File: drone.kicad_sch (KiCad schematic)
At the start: 0 parts

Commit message: Added sensors and mcu
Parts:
- added J1: Battery-Banana-Plug-Connector, symbol Connector_Generic:Conn_01x02
- added J10: GPIO7 TH, symbol Connector_Generic:Conn_01x01
- added J11, J12, J13, J14, J15, J16, J17, J18, J19, J20, J8: Conn_01x01, symbol Connector_Generic:Conn_01x01
- added J2: AF-MPM3610-Converter, Adafruit MPM3610:1X04_ROUND, symbol Adafruit MPM3610-eagle-import:HEADER-1X4ROUND
- added J21: GPIO9_TH, symbol Connector_Generic:Conn_01x01
- added J22: GPIO8 TH, symbol Connector_Generic:Conn_01x01
- added J3: ESC_1, symbol Connector_Generic:Conn_01x01
- added J4: ESC_2, symbol Connector_Generic:Conn_01x01
- added J5, J6: ESC_3, symbol Connector_Generic:Conn_01x01
- added J7: VCC_MCU_Sensors, symbol Connector_Generic:Conn_01x01
- added J9: GPIO44 TH, symbol Connector_Generic:Conn_01x01
- added S1: AF-QMC5883P-Magnetometer, Adafruit QMC5883P Magnetometer:1X05_ROUND_70, symbol Adafruit QMC5883P Magnetometer-eagle-import:HEADER-1X570MIL
- added S2: AF-BMP280-Barometer, Adafruit BMP280:1X07_ROUND_70, symbol Adafruit BMP280-eagle-import:HEADER-1X770MIL
- added S3: AF-MPU6050-Accel/Gyro, Adafruit MPU6050:1X06_ROUND_70, symbol Adafruit MPU6050-eagle-import:HEADER-1X670MIL
- added S4: AF-MPU6050-Accel/Gyro, Adafruit MPU6050:1X06_ROUND, symbol Adafruit MPU6050-eagle-import:HEADER-1X6ROUND
- added U1, U2: ESP32-S3, symbol Adafruit BMP280-eagle-import:HEADER-1X770MIL
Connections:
- new net: J14.1 (Pin_1), S4.4
- new net 3Vo: S1.2, S2.2, S3.2
- new net 5VIN: U1.1
- new net AD0: J11.1 (Pin_1), S4.1
- new net CLKIN: J15.1 (Pin_1), S4.5
- new net CS_5V: S2.7
- new net EN: J2.1
- new net FSYNC_IN: J12.1 (Pin_1), S4.2
- new net GND: J1.2 (Pin_2), J2.4, S1.3, S2.3, S3.3, S4.6, U1.2
- new net GPIO1: J16.1 (Pin_1), U2.1
- new net GPIO2: J17.1 (Pin_1), U2.2
- new net GPIO3: J18.1 (Pin_1), U2.3
- new net GPIO4: J19.1 (Pin_1), U2.4
- new net GPIO43: J20.1 (Pin_1), S1.4, S2.4, S3.4, U2.6, U2.7
- new net GPIO44: J9.1 (Pin_1), U1.7
- new net GPIO7: J10.1 (Pin_1), U1.6
- new net GPIO8: J22.1 (Pin_1), U1.5
- new net GPIO9: J21.1 (Pin_1), U1.4
- new net INT: S3.6
- new net SCL_EXT: J13.1 (Pin_1), S4.3
- new net SDA: S1.5, S2.6, S3.5, U2.5
- new net SDO/ADR_3V: S2.5
- new net VBat: J1.1 (Pin_1), J2.2, J3.1 (Pin_1), J4.1 (Pin_1), J5.1 (Pin_1), J6.1 (Pin_1)
- new net VCC_3V3: J2.3, J8.1 (Pin_1)
- new net VCC_3V3_MCU: J7.1 (Pin_1), S1.1, S2.1, S3.1, U1.3

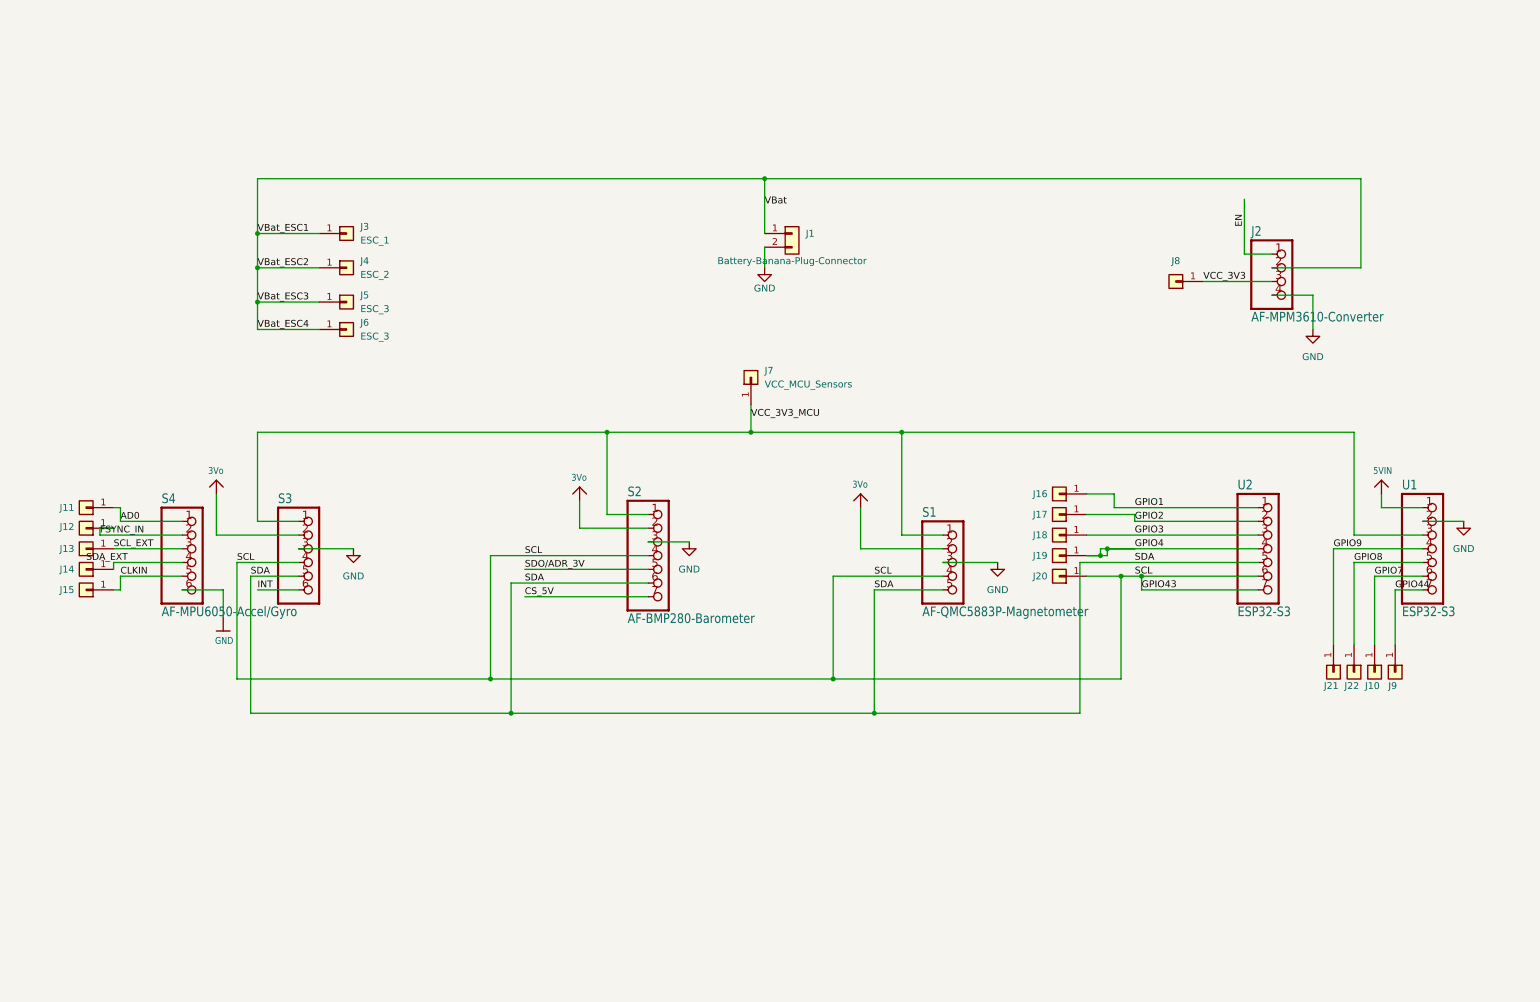
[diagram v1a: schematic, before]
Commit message: Initial commit 2
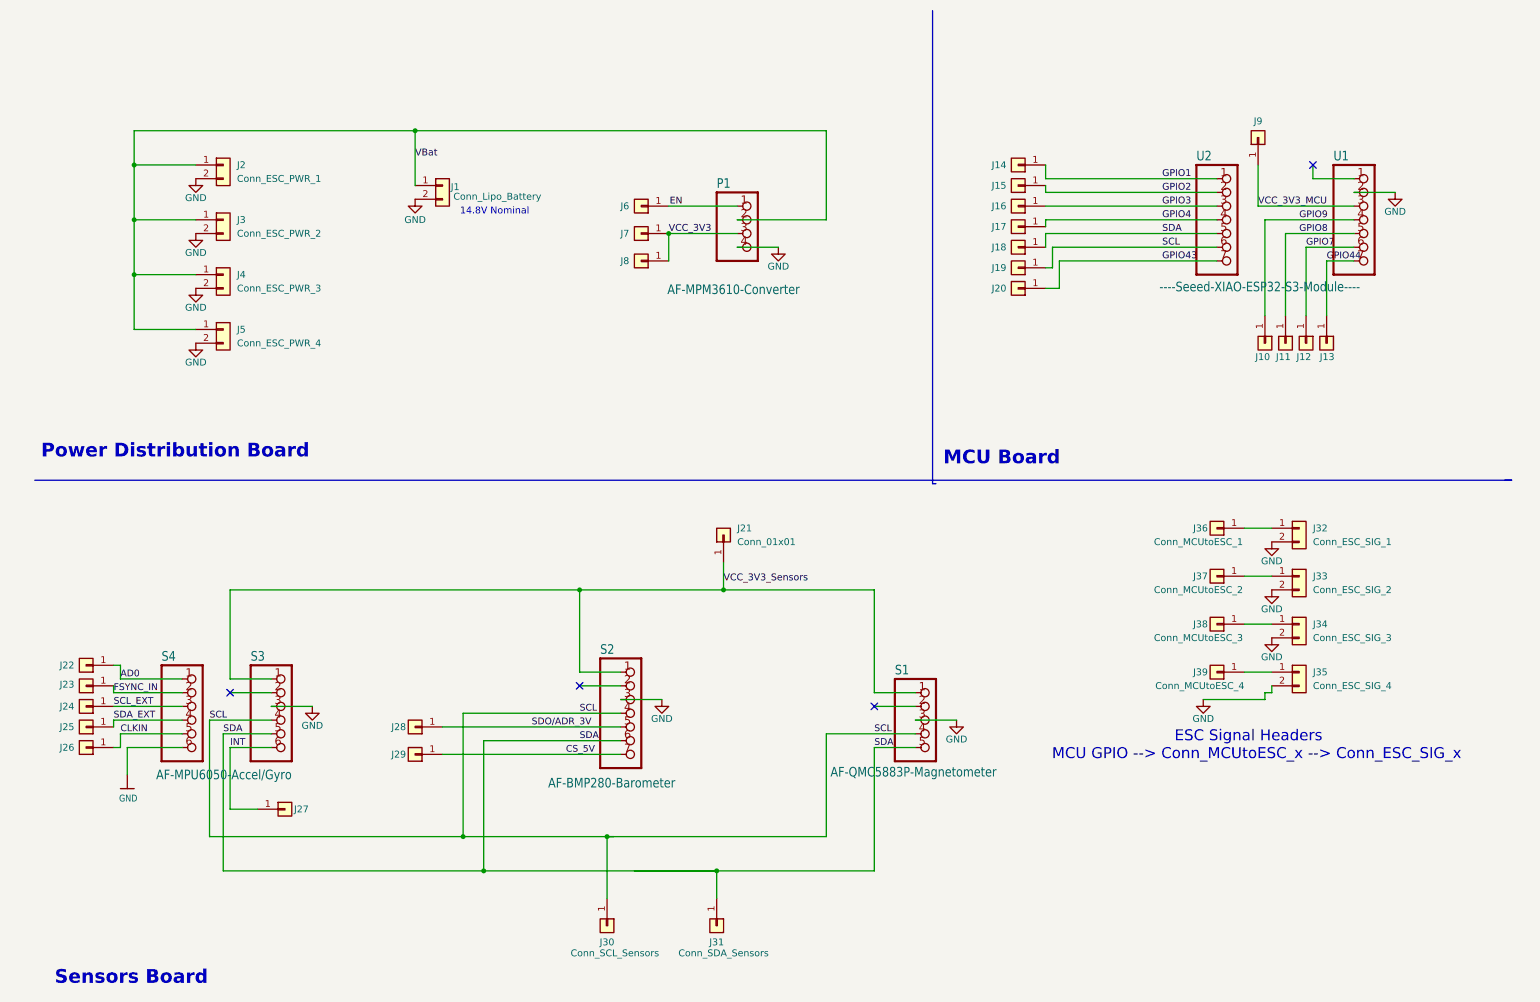
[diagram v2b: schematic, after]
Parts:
- removed J3: ESC_1, symbol Connector_Generic:Conn_01x01
- removed J4: ESC_2, symbol Connector_Generic:Conn_01x01
- removed J5: ESC_3, symbol Connector_Generic:Conn_01x01
- added J18, J20, J27, J28, J29, J8, J9: Conn_01x01, symbol Connector_Generic:Conn_01x01
- added J2: Conn_ESC_PWR_1, symbol Connector_Generic:Conn_01x02
- added J3: Conn_ESC_PWR_2, symbol Connector_Generic:Conn_01x02
- added J30: Conn_SCL_Sensors, symbol Connector_Generic:Conn_01x01
- added J31: Conn_SDA_Sensors, symbol Connector_Generic:Conn_01x01
- added J32: Conn_ESC_SIG_1, symbol Connector_Generic:Conn_01x02
- added J33: Conn_ESC_SIG_2, symbol Connector_Generic:Conn_01x02
- added J34: Conn_ESC_SIG_3, symbol Connector_Generic:Conn_01x02
- added J35: Conn_ESC_SIG_4, symbol Connector_Generic:Conn_01x02
- added J36: Conn_MCUtoESC_1, symbol Connector_Generic:Conn_01x01
- added J37: Conn_MCUtoESC_2, symbol Connector_Generic:Conn_01x01
- added J38: Conn_MCUtoESC_3, symbol Connector_Generic:Conn_01x01
- added J39: Conn_MCUtoESC_4, symbol Connector_Generic:Conn_01x01
- added J4: Conn_ESC_PWR_3, symbol Connector_Generic:Conn_01x02
- added J5: Conn_ESC_PWR_4, symbol Connector_Generic:Conn_01x02
- J1: value Battery-Banana-Plug-Connector -> Conn_Lipo_Battery
- J21: renamed from J7; value VCC_MCU_Sensors -> Conn_01x01
- J6: value ESC_3 -> Conn_01x01
- U1: value ESP32-S3 -> ----Seeed-XIAO-ESP32-S3-Module----
- renumbered J21 to J10, J22 to J11, J10 to J12, J9 to J13, J16 to J14, J17 to J15, J18 to J16, J19 to J17, J20 to J19, J11 to J22, J12 to J23, J13 to J24, J14 to J25, J15 to J26, J8 to J7, J2 to P1
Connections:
- net CS_5V: now also J29.1 (Pin_1)
- net EN: now also J6.1 (Pin_1)
- net GND: now also J2.2 (Pin_2), J3.2 (Pin_2), J32.2 (Pin_2), J33.2 (Pin_2), J34.2 (Pin_2), J35.2 (Pin_2), J4.2 (Pin_2), J5.2 (Pin_2)
- net GPIO43: now also J20.1 (Pin_1); no longer J19.1 (Pin_1), S1.4, S2.4, S3.4, U2.6
- net INT: now also J27.1 (Pin_1)
- net SDA: now also J18.1 (Pin_1), J31.1 (Pin_1)
- net SDA_EXT: now also J25.1 (Pin_1), S4.4
- net SDO/ADR_3V: now also J28.1 (Pin_1)
- net VBat: now also J2.1 (Pin_1), J3.1 (Pin_1), J4.1 (Pin_1), J5.1 (Pin_1); no longer J6.1 (Pin_1)
- net VCC_3V3: now also J8.1 (Pin_1)
- net VCC_3V3_MCU: now also J9.1 (Pin_1); no longer J21.1 (Pin_1), S1.1, S2.1, S3.1
- removed net 3Vo: S1.2, S2.2, S3.2
- net 5VIN: no longer names the net of U1.1
- new net: J35.1 (Pin_1), J39.1 (Pin_1)
- new net: J33.1 (Pin_1), J37.1 (Pin_1)
- new net: J32.1 (Pin_1), J36.1 (Pin_1)
- new net: J34.1 (Pin_1), J38.1 (Pin_1)
- new net SCL: J19.1 (Pin_1), J30.1 (Pin_1), S1.4, S2.4, S3.4, U2.6
- new net VCC_3V3_Sensors: J21.1 (Pin_1), S1.1, S2.1, S3.1
- no-connect marks 0 -> 4
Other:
- note added: "14.8V Nominal"
- note added: "ESC Signal Headers"
- note added: "MCU Board"
- note added: "MCU GPIO --> Conn_MCUtoESC_x --> Conn_ESC_SIG_x"
- note added: "Power Distribution Board"
- note added: "Sensors Board"
- moved on the sheet: J1, J10, J11, J12, J13, J14, J15, J16, J17, J19, J21, J22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
